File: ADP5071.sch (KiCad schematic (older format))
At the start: 29 parts, among them P7 PIN, P8 POUT, T1 NET-TIE, U4 ADP5071

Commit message: Latest power stuff
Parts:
- P7: footprint Pin_Headers:Pin_Header_Angled_1x02 -> Pin_Headers:Pin_Header_Straight_1x02
- P8: footprint Pin_Headers:Pin_Header_Angled_1x03 -> Pin_Headers:Pin_Header_Straight_1x03
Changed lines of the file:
@@
 F 0 "P7" H 2000 2900 50  0000 C CNN
 F 1 "PIN" V 2100 2750 50  0000 C CNN
-F 2 "Pin_Headers:Pin_Header_Angled_1x02" H 2000 2750 60  0001 C CNN
+F 2 "Pin_Headers:Pin_Header_Straight_1x02" H 2000 2750 60  0001 C CNN
 F 3 "" H 2000 2750 60  0000 C CNN
 	1    2000 2750
@@
 F 0 "P8" H 9800 3500 50  0000 C CNN
 F 1 "POUT" V 9900 3300 50  0000 C CNN
-F 2 "Pin_Headers:Pin_Header_Angled_1x03" H 9800 3300 60  0001 C CNN
+F 2 "Pin_Headers:Pin_Header_Straight_1x03" H 9800 3300 60  0001 C CNN
 F 3 "" H 9800 3300 60  0000 C CNN
 	1    9800 3300

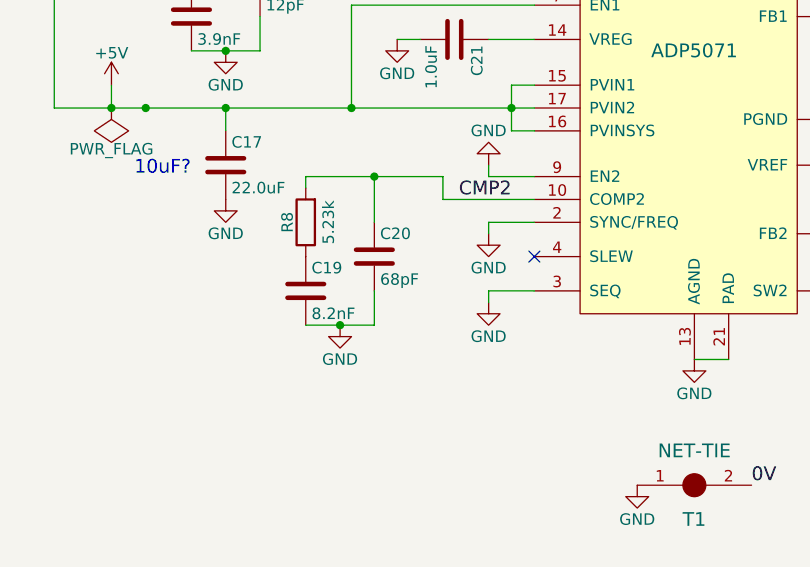
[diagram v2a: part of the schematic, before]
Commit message: Latest work
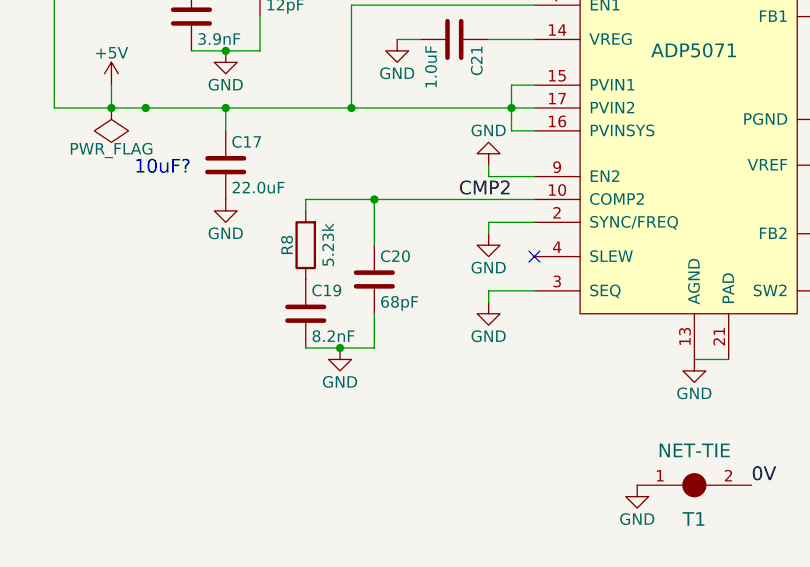
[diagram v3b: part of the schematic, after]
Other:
- moved on the sheet: C19, C20, R8
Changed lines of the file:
@@
 L R R8
 U 1 1 56322611
-P 3700 3800
-F 0 "R8" V 3780 3800 50  0000 C CNN
-F 1 "5.23k" V 3600 3800 50  0000 C CNN
-F 2 "smd:SM0603" V 3630 3800 30  0001 C CNN
-F 3 "" H 3700 3800 30  0000 C CNN
-	1    3700 3800
+P 3700 3900
+F 0 "R8" V 3780 3900 50  0000 C CNN
+F 1 "5.23k" V 3600 3900 50  0000 C CNN
+F 2 "smd:SM0603" V 3630 3900 30  0001 C CNN
+F 3 "" H 3700 3900 30  0000 C CNN
+	1    3700 3900
 	-1   0    0    1
 $EndComp
@@
 L C C19
 U 1 1 56322618
-P 3700 4100
-F 0 "C19" H 3725 4200 50  0000 L CNN
-F 1 "8.2nF" H 3725 4000 50  0000 L CNN
-F 2 "smd:SM0603" H 3738 3950 30  0001 C CNN
-F 3 "" H 3700 4100 60  0000 C CNN
-	1    3700 4100
+P 3700 4200
+F 0 "C19" H 3725 4300 50  0000 L CNN
+F 1 "8.2nF" H 3725 4100 50  0000 L CNN
+F 2 "smd:SM0603" H 3738 4050 30  0001 C CNN
+F 3 "" H 3700 4200 60  0000 C CNN
+	1    3700 4200
 	1    0    0    -1
 $EndComp
@@
 L GND #PWR025
 U 1 1 5632261F
-P 3850 4250
-F 0 "#PWR025" H 3850 4000 50  0001 C CNN
-F 1 "GND" H 3850 4100 50  0000 C CNN
-F 2 "" H 3850 4250 60  0000 C CNN
-F 3 "" H 3850 4250 60  0000 C CNN
-	1    3850 4250
-	1    0    0    -1
-$EndComp
-Wire Wire Line
-	4300 3700 4700 3700
+P 3850 4350
+F 0 "#PWR025" H 3850 4100 50  0001 C CNN
+F 1 "GND" H 3850 4200 50  0000 C CNN
+F 2 "" H 3850 4350 60  0000 C CNN
+F 3 "" H 3850 4350 60  0000 C CNN
+	1    3850 4350
+	1    0    0    -1
+$EndComp
+Wire Wire Line
+	3700 3700 4700 3700
 Wire Wire Line
 	4700 3800 4500 3800
@@
 L C C20
 U 1 1 56322737
-P 4000 3950
-F 0 "C20" H 4025 4050 50  0000 L CNN
-F 1 "68pF" H 4025 3850 50  0000 L CNN
-F 2 "smd:SM0603" H 4038 3800 30  0001 C CNN
-F 3 "" H 4000 3950 60  0000 C CNN
-	1    4000 3950
-	1    0    0    -1
-$EndComp
-Wire Wire Line
-	3700 3650 3700 3600
-Wire Wire Line
-	3700 3600 4300 3600
-Wire Wire Line
-	4300 3600 4300 3700
-Wire Wire Line
-	4000 3800 4000 3600
-Connection ~ 4000 3600
-Wire Wire Line
-	3700 4250 4000 4250
-Wire Wire Line
-	4000 4250 4000 4100
-Connection ~ 3850 4250
+P 4000 4050
+F 0 "C20" H 4025 4150 50  0000 L CNN
+F 1 "68pF" H 4025 3950 50  0000 L CNN
+F 2 "smd:SM0603" H 4038 3900 30  0001 C CNN
+F 3 "" H 4000 4050 60  0000 C CNN
+	1    4000 4050
+	1    0    0    -1
+$EndComp
+Wire Wire Line
+	3700 3750 3700 3700
+Wire Wire Line
+	4000 3900 4000 3700
+Connection ~ 4000 3700
+Wire Wire Line
+	3700 4350 4000 4350
+Wire Wire Line
+	4000 4350 4000 4200
+Connection ~ 3850 4350
 $Comp
 L R R13
